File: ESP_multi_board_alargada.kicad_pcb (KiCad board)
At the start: 2 copper layers, 24 parts, among them P101 CONN_01X02, P102 CONN_01X06, P103 CONN_01X02, P104 CONN_01X06, P105 CONN_01X12, P106 CONN_01X03, P107 CONN_I2C_MPU6050, P108 CONN_PINES_DIG, SW101 SW_PUSH_SMALL, SW102 SWITCH_INV, U1 LD1117S33TR, U101 L293DD, U102 ESP-12, U103 MAX11605EEE+, U104 MCP23008

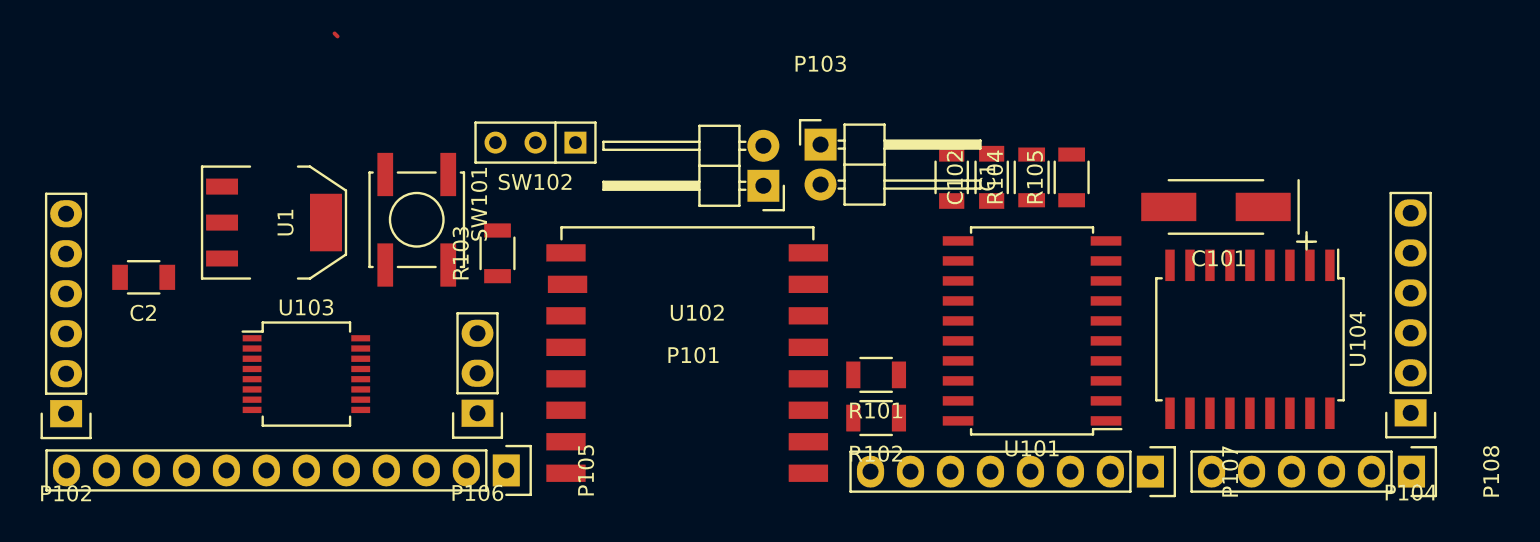
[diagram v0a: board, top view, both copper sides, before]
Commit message: routing
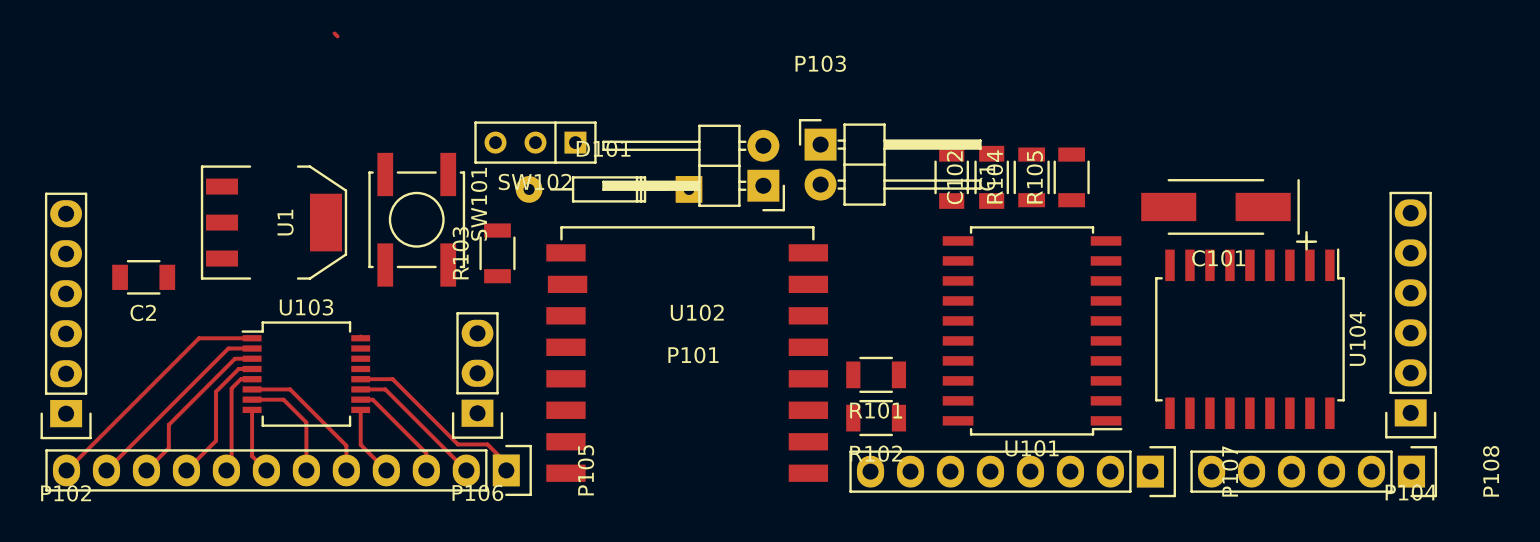
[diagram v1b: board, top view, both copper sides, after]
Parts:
- added D101: D, Diodes_ThroughHole:Diode_DO-35_SOD27_Horizontal_RM10, F.Cu at (167.1, 75.9)
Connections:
- P101 pad 2: Net-(P101-Pad2) -> Net-(D101-Pad1)
- SW102 pad 2: Net-(P101-Pad2) -> Net-(D101-Pad2)
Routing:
- net Net-(P105-Pad12): track 0.00 -> 15.3 mm
- net Net-(P105-Pad11): track 0.00 -> 12.5 mm
- net Net-(P105-Pad1): track 0.00 -> 11.9 mm
- net Net-(P105-Pad10): track 0.00 -> 10.5 mm
- net Net-(P105-Pad5): track 0.00 -> 9.04 mm
- net Net-(P105-Pad2): track 0.00 -> 8.84 mm
- net Net-(P105-Pad9): track 0.00 -> 8.67 mm
- net Net-(P105-Pad6): track 0.00 -> 7.10 mm
- net Net-(P105-Pad8): track 0.00 -> 6.89 mm
- net Net-(P105-Pad3): track 0.00 -> 6.67 mm
- net Net-(P105-Pad4): track 0.00 -> 4.52 mm
- net Net-(P105-Pad7): track 0.00 -> 4.22 mm
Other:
- net class Default: trace_width 0.25 -> 0.3
- net class power: trace_width 0.25 -> 0.3
- net class small added: clearance 0.25, trace_width 0.25, via_dia 0.6, via_drill 0.4
- net class special added: clearance 0.2, trace_width 0.3, via_dia 0.6, via_drill 0.4
- net class special+ added: clearance 0.15, trace_width 0.3, via_dia 0.6, via_drill 0.4
